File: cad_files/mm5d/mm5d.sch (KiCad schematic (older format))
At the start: 12 parts, among them P1 SCREW_CONN_1, P2 SCREW_CONN_1, P3 SCREW_CONN_1, P37 DB9, P4 CONN_02X20, P5 CONN_02X20, P6 CONN_02X20, U3 Matrix_display, U6 Relay_panel, U7 Relay_panel

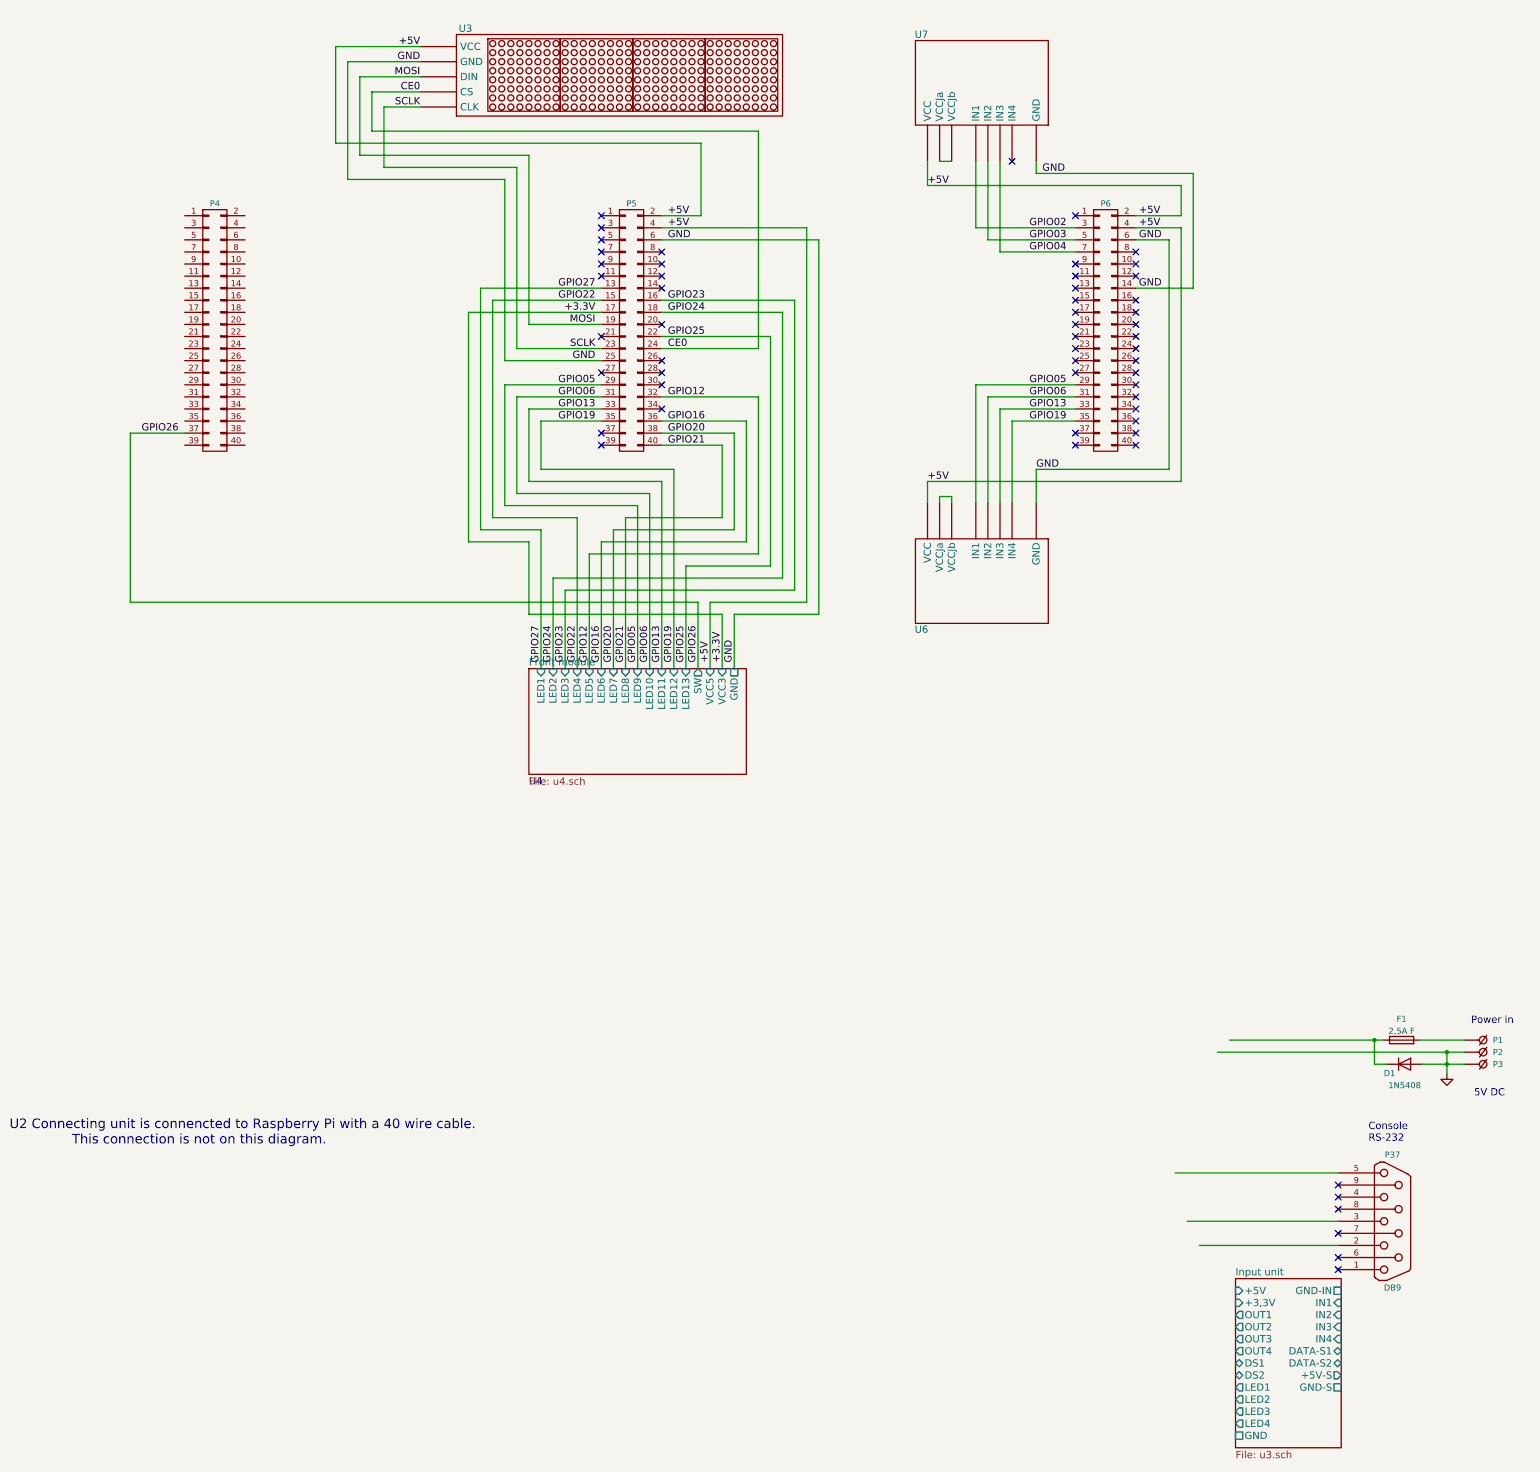
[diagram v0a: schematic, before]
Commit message: 200129
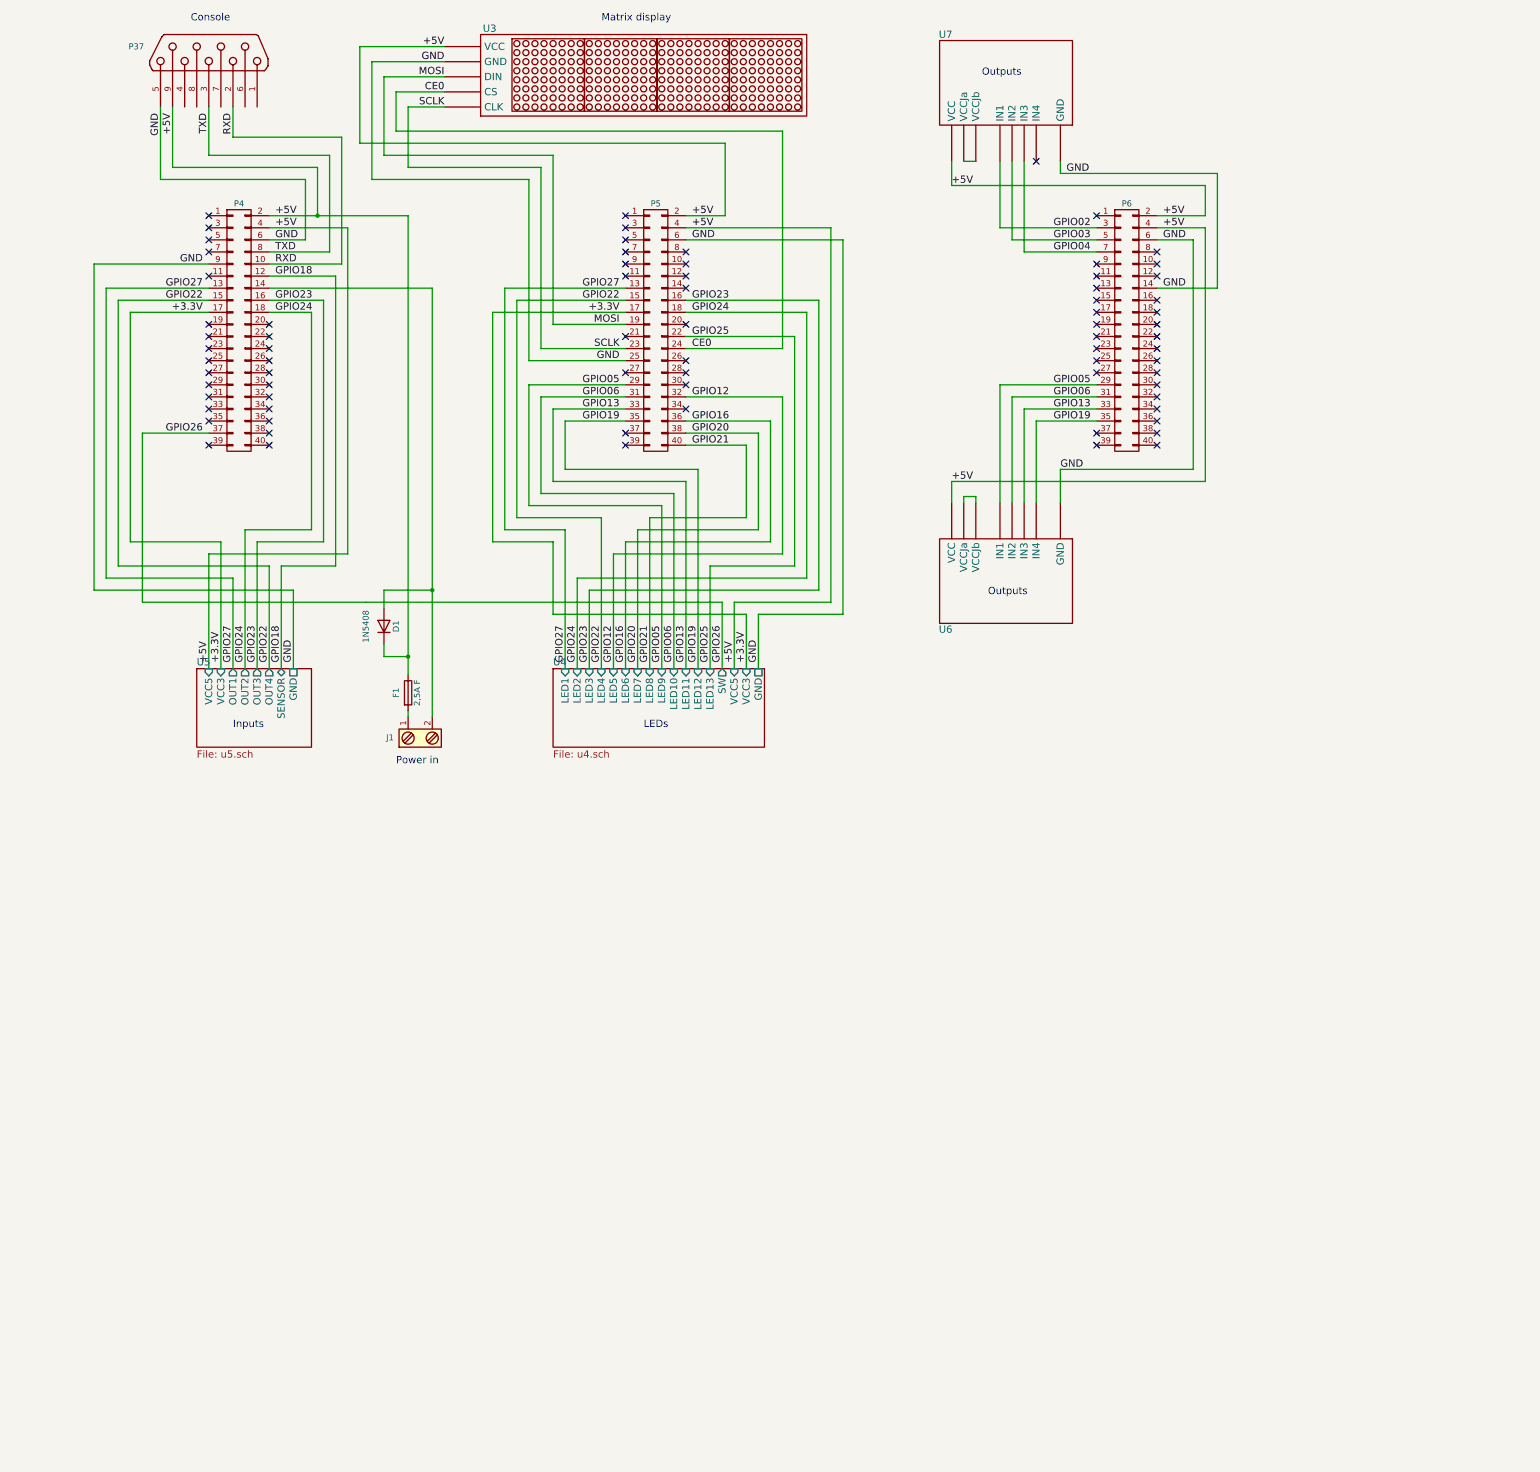
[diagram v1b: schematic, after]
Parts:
- removed P1, P2, P3: SCREW_CONN_1, symbol SCREW_CONN_1
- added J1: Screw_Terminal_1x02, symbol Screw_Terminal_1x02
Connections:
- net labels added: GPIO18, RXD, TXD
- wire segments 139 -> 189
- no-connect marks 55 -> 75
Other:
- note added: "Console"
- note added: "Inputs"
- note added: "LEDs"
- note added: "Matrix display"
- note added: "Outputs"
- note removed: "5V DC"
- note removed: "Console\nRS-232"
- note removed: "U2 Connecting unit is connencted to Raspberry Pi with a 40 wire cable.\n This connection is not on this diagram."
- note removed: "U4"
- moved on the sheet: D1, F1, P37, P4, P5, P6, U3, U6, U7
